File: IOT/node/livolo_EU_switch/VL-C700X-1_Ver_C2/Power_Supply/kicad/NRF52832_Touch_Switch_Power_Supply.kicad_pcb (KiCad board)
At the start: 2 copper layers, 46 x 43.4 mm, 56 parts, among them CN1 2X7P, K1 HFE60-12-1HT-L2, K2 HFE60-12-1HT-L2, Q1 IRLR8726PBF, Q2 MMBT3904, T1 EE10A-1, U1 LM321, U2 MCP1703T-3302, U3 EL357, U4 LNK364DN-TL, U6 TPL7407LPWR

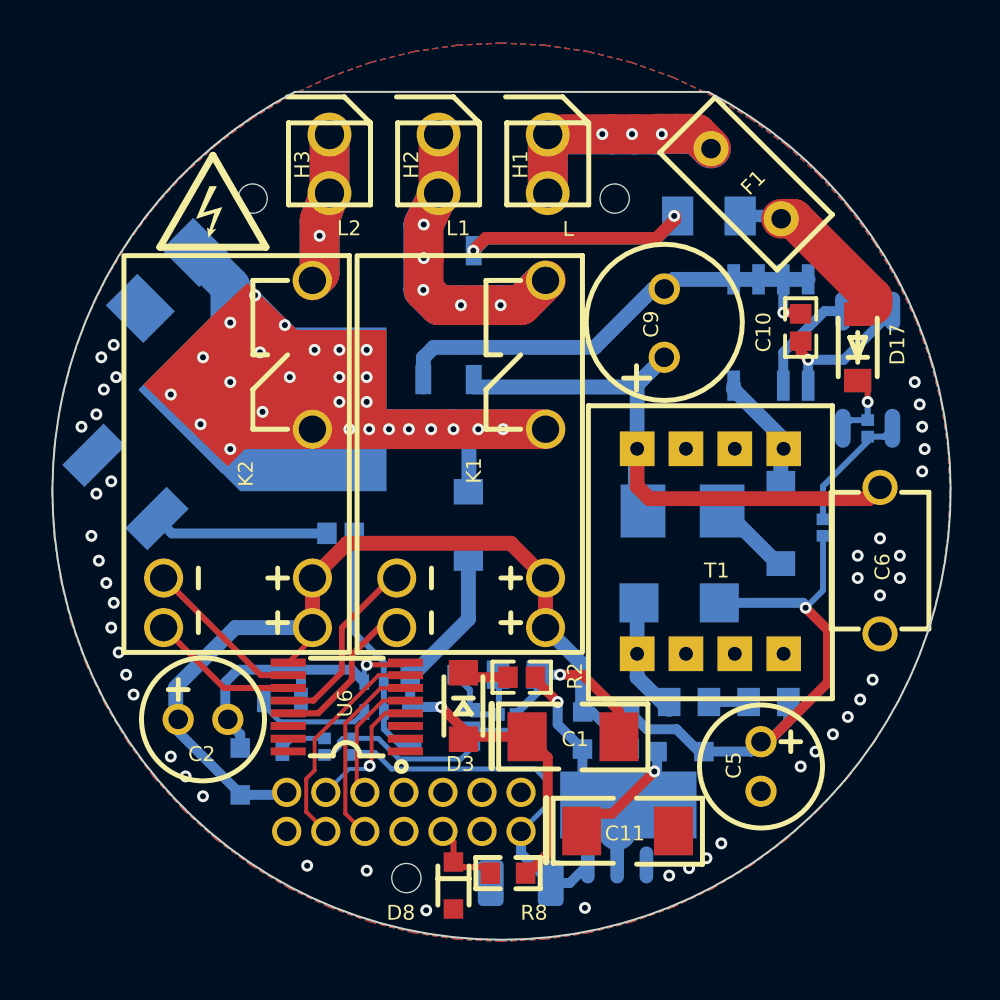
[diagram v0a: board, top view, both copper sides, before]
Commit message: eu switch rev0.4 - the last one
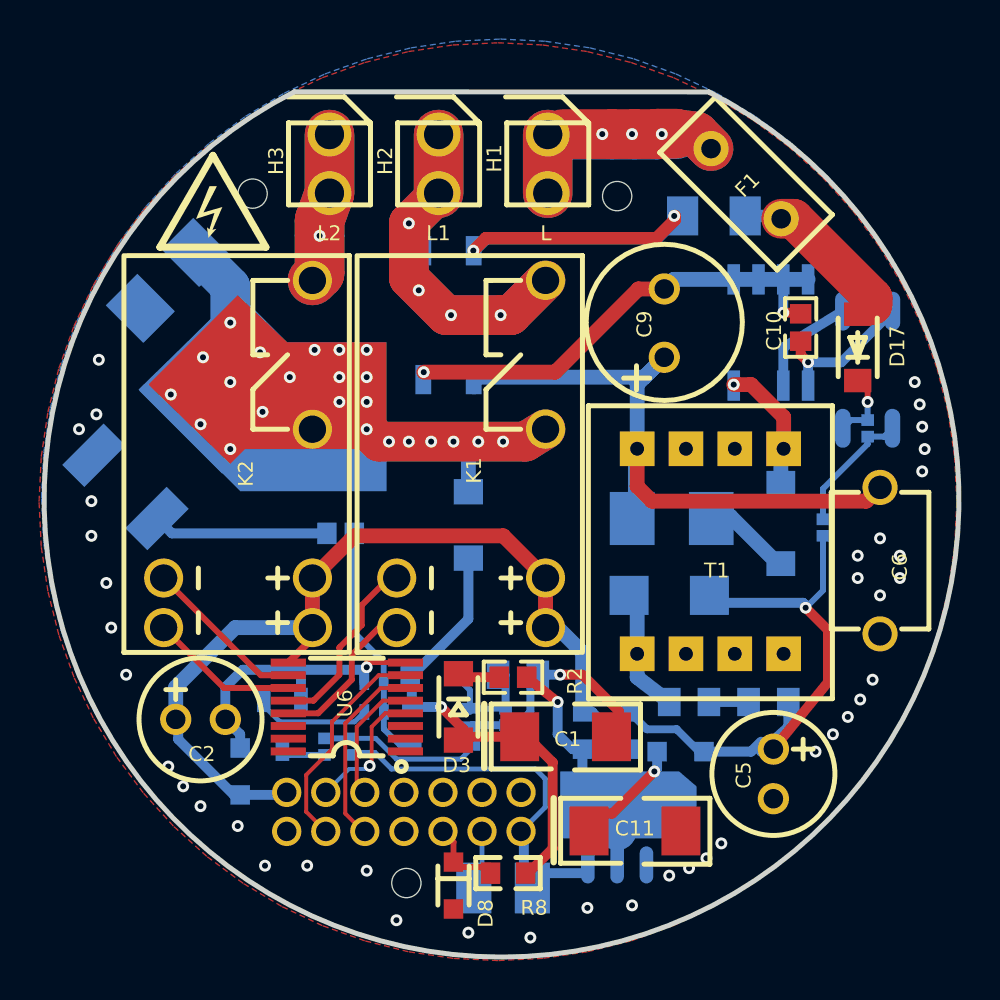
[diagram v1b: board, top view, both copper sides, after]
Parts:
- removed REF** (x3): MountingHole_2mm, MountingHole:MountingHole_2mm
- added ?: , AutoGenerated:MountingHole_1.50mm, F.Cu at (120.8, 43.3)
- added ?: , AutoGenerated:MountingHole_1.50mm, F.Cu at (102.1, 43.2)
- added ?: , AutoGenerated:MountingHole_1.50mm, F.Cu at (110.0, 78.5)
- C3: value 22uF -> CAP-SMD_L3.5-W2.8-R-RD; footprint Capacitor_Tantalum_SMD:CP_EIA-3528-21_Kemet-B -> easyeda:CAP-SMD_L3.5-W2.8-R-RD; moved to F.Cu
- moved C3 0.94 mm to (114.9, 78.7), turned to 180 degrees
- moved C5 0.74 mm to (128.8, 72.9)
- moved D15 0.67 mm to (123.6, 59.8)
- moved D14 0.64 mm to (123.4, 63.8)
- moved R2 0.45 mm to (115.4, 67.9)
- moved C1 0.38 mm to (118.2, 71.0)
- moved C11 0.38 mm to (121.8, 75.8)
- moved D3 0.26 mm to (112.6, 69.5)
- moved R20 0.25 mm to (125.7, 44.3)
- moved R7 0.15 mm to (115.1, 70.0), turned to 270 degrees
- moved C2 0.13 mm to (99.4, 70.1)
- turned R3 to 270 degrees
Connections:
- C3 pad 1: GND -> +3V3
- C3 pad 2: +3V3 -> GND
- C7 pad 1: (no net) -> R16_2
- D13 pad 2: (no net) -> D13_2
- R16 pad 2: (no net) -> R16_2
- R20 pad 2: (no net) -> D13_2
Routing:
- net (no net): track 24.4 -> 0.00 mm, vias 2 -> 0
- net D13_2: track 0.00 -> 22.6 mm, vias 0 -> 2
- net D1_1: track 56.5 -> 45.8 mm, vias 26 -> 23
- net GND: track 36.7 -> 39.3 mm, vias 46 -> 42
- net AC_DC_N: track 30.5 -> 33.0 mm, vias 5 -> 4
- net R16_2: track 0.00 -> 2.03 mm
- net U4_5: track 25.7 -> 24.5 mm, vias 1 -> 2
- net +12V: track 51.7 -> 52.6 mm
- net R2_2: track 19.4 -> 20.0 mm
- net U4_4: track 6.35 -> 6.84 mm, vias 0 -> 1
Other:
- board size 46 x 43.4 mm -> 46.8 x 44.3 mm
- rule pad_to_mask_clearance: 0.051 -> 0
- board text added: "REV. 0.4"
- board text removed: "REV. 0.3"
